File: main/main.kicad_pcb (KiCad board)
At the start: 2 copper layers, 45.1 x 52.6 mm, 37 parts, among them P2 CONN_5, P7 CONN_10, P8 CONN_7, SW1 S01_Socket, SW2 S01_Socket, SW3 S01_Socket, SW4 CMI126603D08, SW6 CMI126603D08, U1 MKL17Z32VFM4, U4 ESD

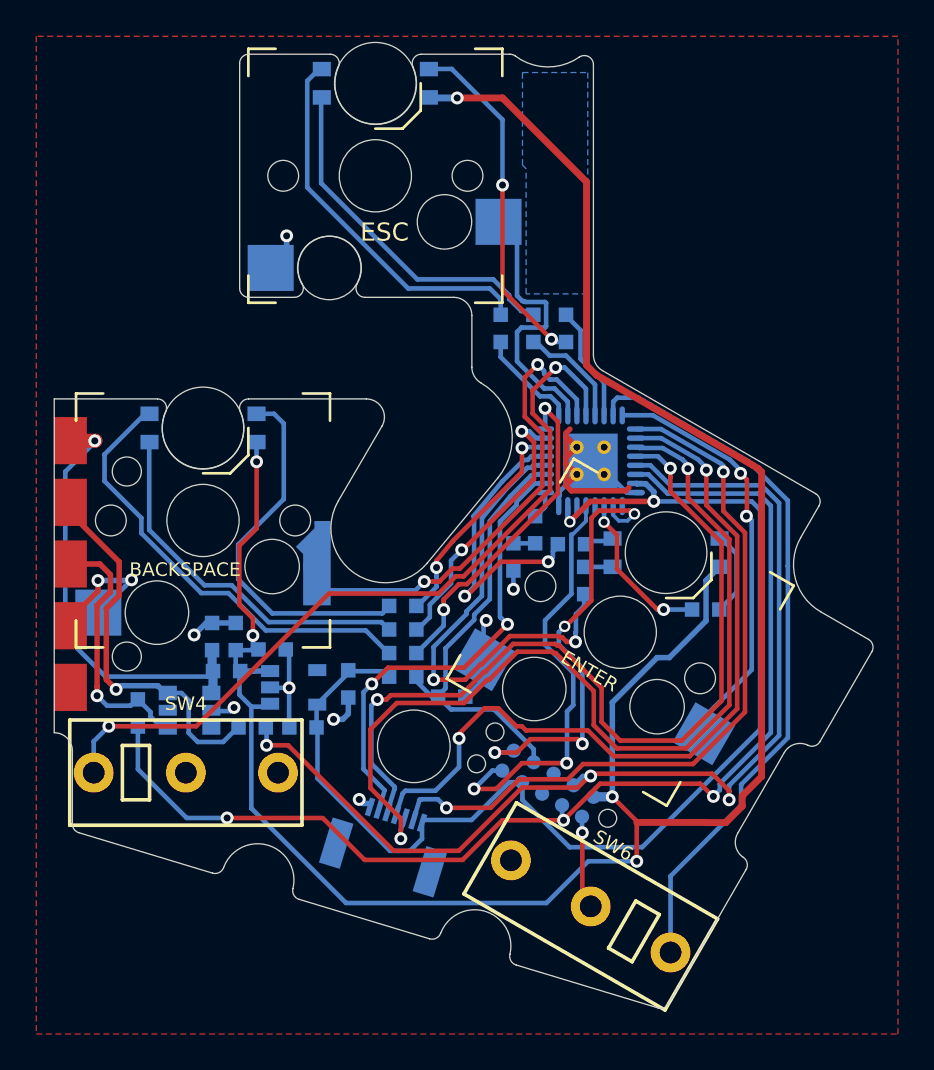
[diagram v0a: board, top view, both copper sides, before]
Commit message: Clean up silk screen.
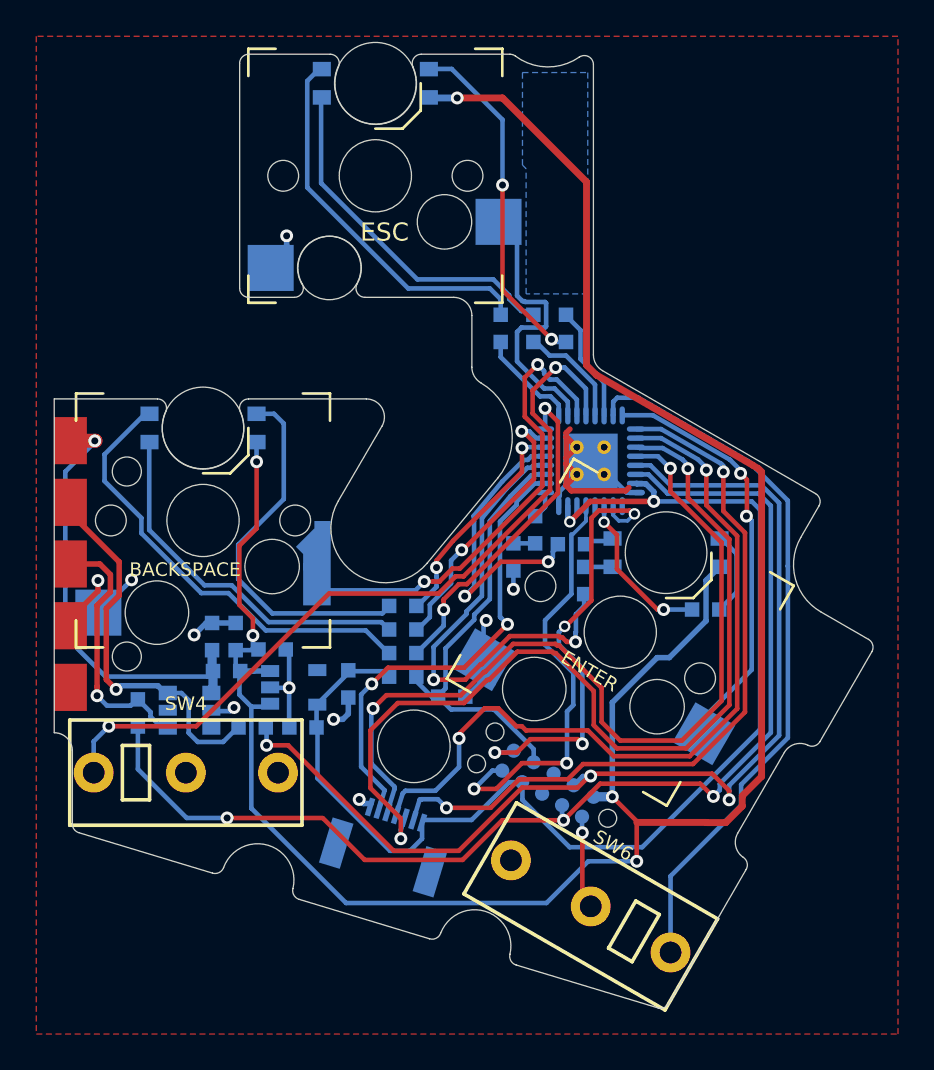
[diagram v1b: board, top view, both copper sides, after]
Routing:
- net GND: track 45.3 -> 44.1 mm
